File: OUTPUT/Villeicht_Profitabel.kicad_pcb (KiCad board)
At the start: 2 copper layers, 25 x 40 mm, 5 parts, among them J1 Conn_01x03_Pin, Q2 QM6006D

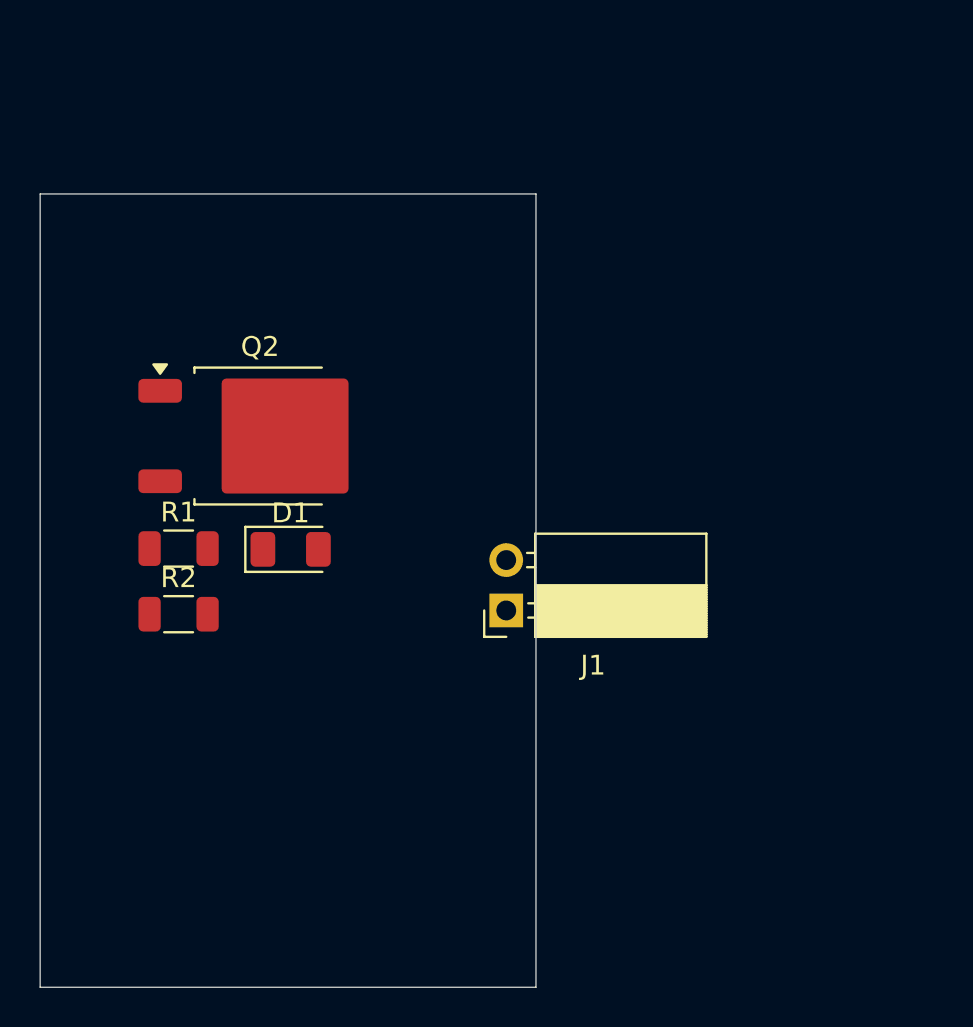
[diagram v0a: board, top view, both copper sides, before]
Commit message: Auto-update: 19.12.2025  7:18:55,05
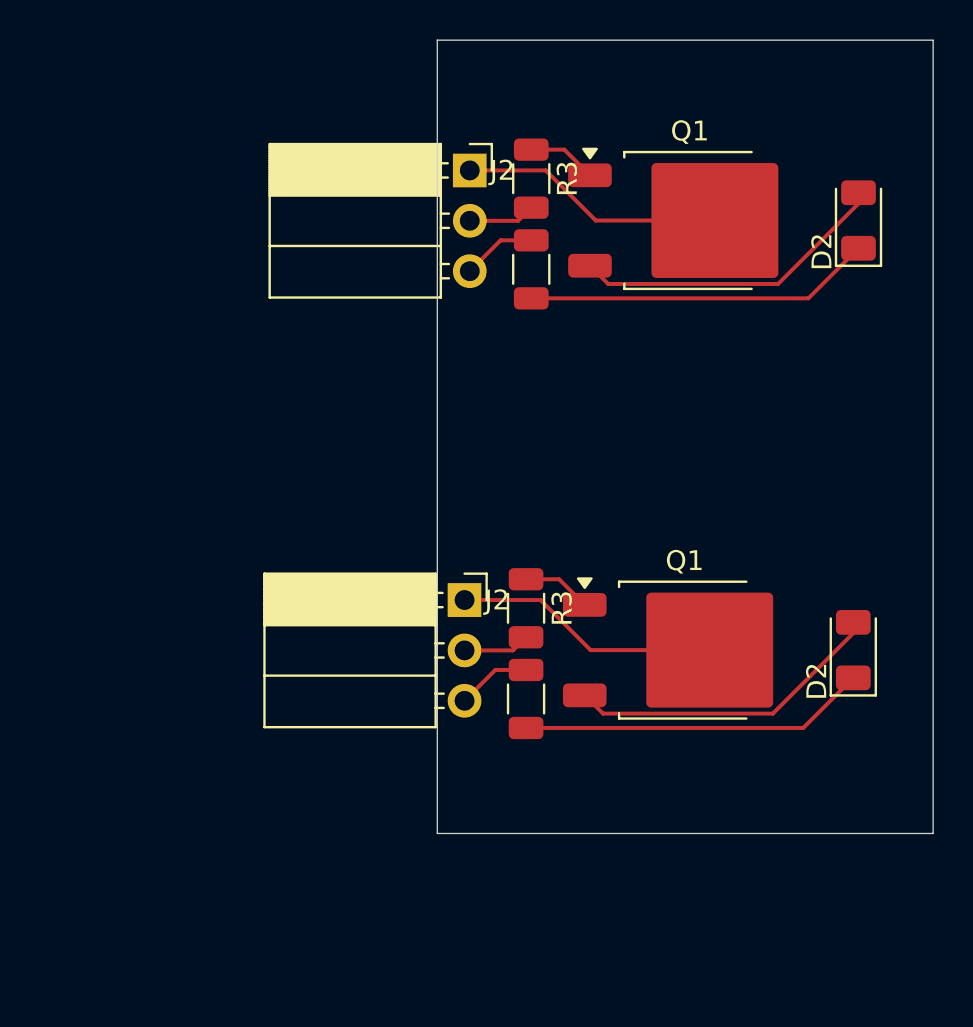
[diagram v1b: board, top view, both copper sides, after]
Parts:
- removed D1: LED, LED_SMD:LED_1206_3216Metric
- removed J1: Conn_01x03_Pin, Connector_PinSocket_2.54mm:PinSocket_1x02_P2.54mm_Horizontal
- removed Q2: QM6006D, Package_TO_SOT_SMD:TO-252-2
- removed R1: R, Resistor_SMD:R_1206_3216Metric
- removed R2: 1k, Resistor_SMD:R_1206_3216Metric
- added D2: LED, LED_SMD:LED_1206_3216Metric, F.Cu at (176.0, 121.0)
- added D2: LED, LED_SMD:LED_1206_3216Metric, F.Cu at (176.3, 99.3)
- added J2: Conn_01x03_Pin, Connector_PinSocket_2.54mm:PinSocket_1x03_P2.54mm_Horizontal, F.Cu at (156.7, 96.8)
- added J2: Conn_01x03_Pin, Connector_PinSocket_2.54mm:PinSocket_1x03_P2.54mm_Horizontal, F.Cu at (156.4, 118.5)
- added Q1: QM6006D, Package_TO_SOT_SMD:TO-252-2, F.Cu at (167.8, 99.3)
- added Q1: QM6006D, Package_TO_SOT_SMD:TO-252-2, F.Cu at (167.5, 121.0)
- added R3: 1k, Resistor_SMD:R_1206_3216Metric, F.Cu at (159.5, 118.9)
- added R3: 1k, Resistor_SMD:R_1206_3216Metric, F.Cu at (159.8, 97.2)
- added R4: R, Resistor_SMD:R_1206_3216Metric, F.Cu at (159.8, 101.8)
- added R4: R, Resistor_SMD:R_1206_3216Metric, F.Cu at (159.5, 123.5)
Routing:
- net Net-(D2-K): track 0.00 -> 35.1 mm
- net Net-(D2-A): track 0.00 -> 32.3 mm
- net Net-(J2-Pin_1): track 0.00 -> 26.8 mm
- net Net-(J2-Pin_3): track 0.00 -> 7.49 mm
- net Net-(Q1-G): track 0.00 -> 6.99 mm
- net Net-(J2-Pin_2): track 0.00 -> 6.75 mm
